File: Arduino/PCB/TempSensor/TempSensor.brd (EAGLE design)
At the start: 40.3 x 30.5 mm, 13 parts, among them IC1 DS18B20, U1 ATMEGA328-AU, X1 16Mhz

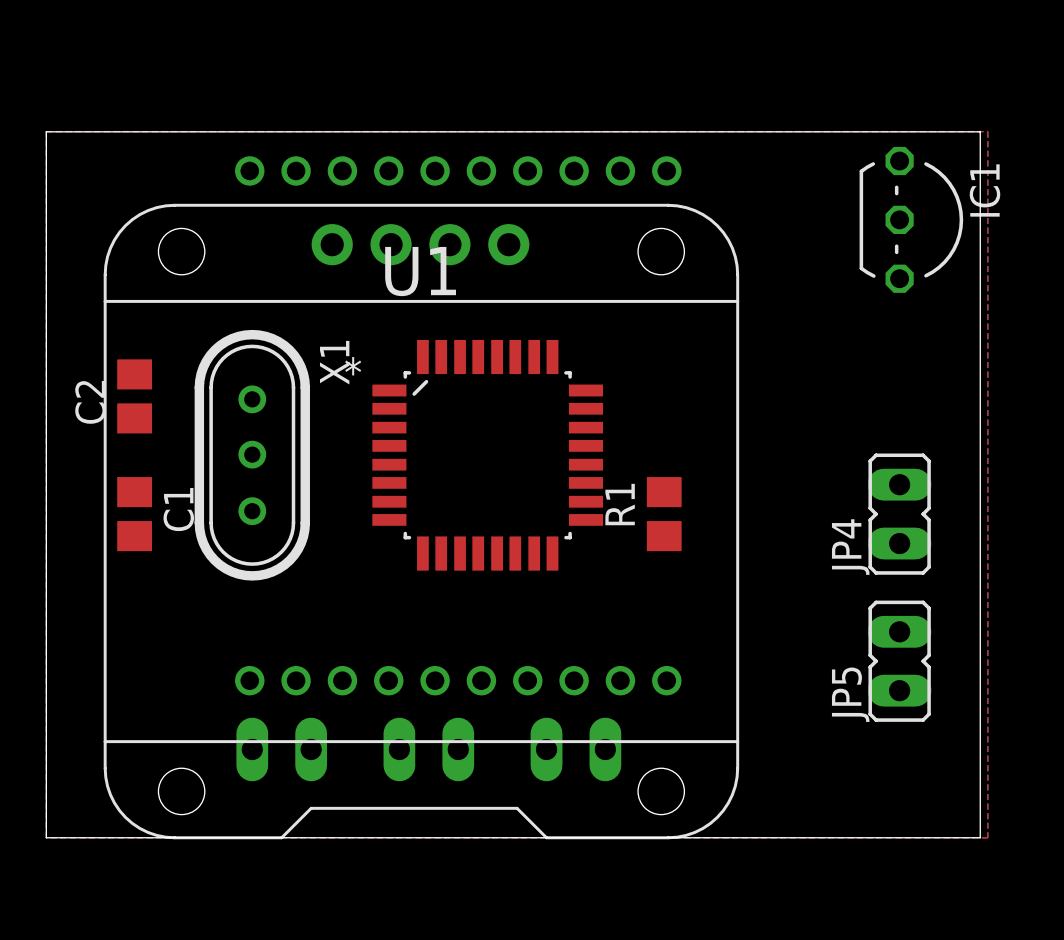
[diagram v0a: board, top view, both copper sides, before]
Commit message: sensor pcb
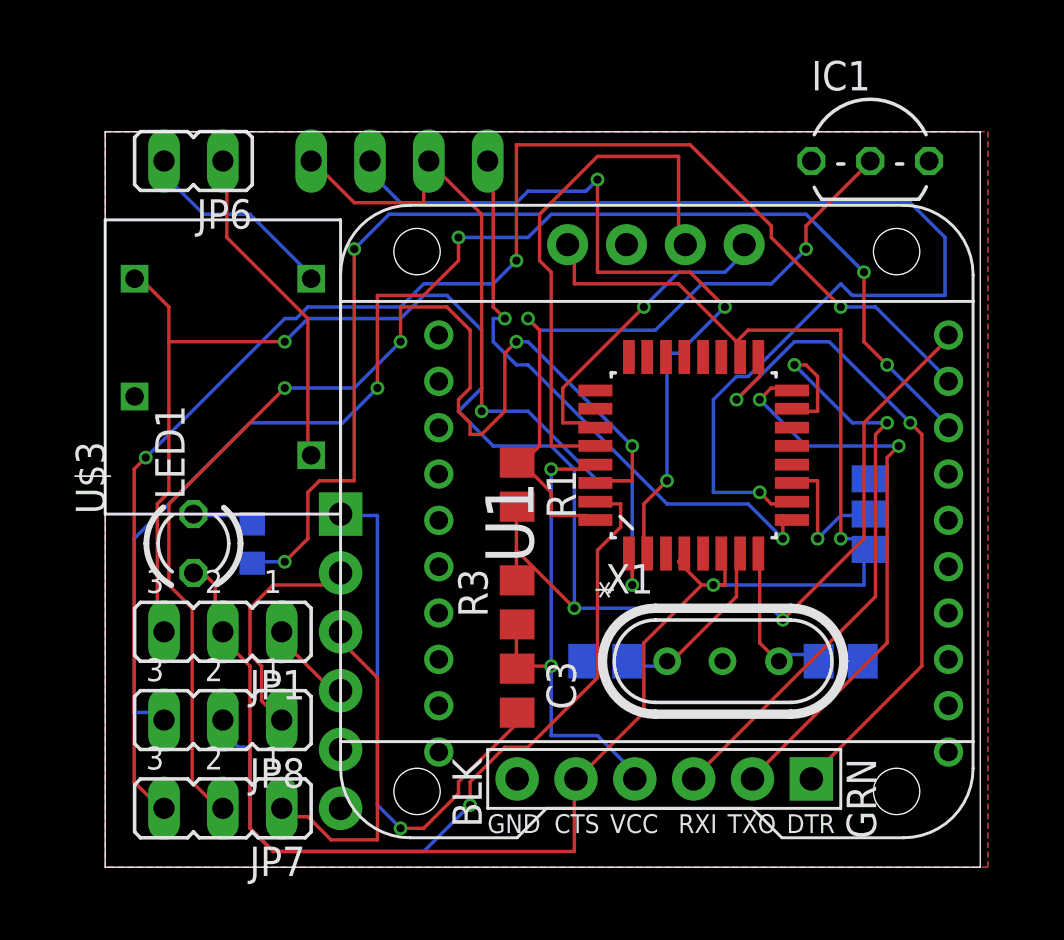
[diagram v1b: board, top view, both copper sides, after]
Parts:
- removed JP2, JP3: (no value), jumper:JP1
- added C3: 100n, rcl:C0805
- added J1, J2: FTDI_DEVICE, SparkFun-Connectors:FTDI_DEVICE_SIDE
- added JP6: (no value), jumper:JP1
- added JP7, JP8: (no value), jumper:JP2
- added LED1: 2mA, led:LED3MM
- added R2: 580, rcl:R0603
- added R3: 10k, rcl:R0805
- added SJ2: (no value), jumper:SJ_2
- added U$3: IE0503D, xp_power:XP_DIP
- JP1: device jumper:JP1 -> jumper:JP2
- R1: value (none) -> 4k7
- moved C1 31.1 mm to (63.5, 29.2), flipped to the bottom, turned to 180 degrees
- moved JP5 28.8 mm to (47.0, 50.8), flipped to the bottom, turned to 90 degrees
- moved JP4 28.5 mm to (41.9, 50.8), flipped to the bottom, turned to 90 degrees
- moved C2 23.3 mm to (53.3, 29.2), flipped to the bottom, turned to 180 degrees
- moved X1 22.2 mm to (58.4, 29.2), turned to 0 degrees
- moved XB1 11.4 mm to (57.1, 34.3), turned to 0 degrees
- moved U$2 10.2 mm to (55.9, 35.6)
- moved U1 8.89 mm to (57.1, 38.1), turned to 90 degrees
- moved R1 6.48 mm to (49.5, 36.8), turned to 270 degrees
- moved JP1 5.68 mm to (36.8, 30.5), flipped to the top, turned to 180 degrees
- moved IC1 2.84 mm to (64.8, 50.8), turned to 0 degrees
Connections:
- removed net N$3: JP3.2, XB1.1
- new net +5V: J1.P$4, JP1.1
- new net N$11: JP6.2, U$3.+VIN
- new net N$14: JP6.1, U$3.-VIN
- new net N$15: LED1.K, R2.2
- new net N$16: R2.1, U1.10
- new net N$17: SJ2.2, U1.11
- new net N$18: JP7.3, XB1.2
- new net N$19: JP8.3, XB1.3
- new net N$20: C3.1, J2.P$4, R3.1, U1.29
- new net N$21: C3.2, J1.P$1
- new net N$22: J2.P$3, U1.15
- new net N$23: J2.P$1, U1.17
- new net N$24: J2.P$2, U1.16
- new net VCC: J2.P$5, JP1.2, LED1.A, SJ2.1, U$2.VCC, U1.18, U1.4, U1.6
- net +3V3: now also JP1.3, R3.2, U$3.+VOUT, XB1.1; no longer JP3.1, U$2.VCC, U1.18, U1.4, U1.6
- net GND: now also J1.P$6, J2.P$6, SJ2.3, U$3.-VOUT
- net N$4: now also JP7.2; no longer JP1.1
- net N$5: now also JP8.2, U1.31; no longer JP1.2, XB1.2
- net N$6: now also J1.P$3, JP7.1; no longer JP2.1, XB1.3
- net N$7: now also J1.P$2, JP8.1; no longer JP2.2, U1.31
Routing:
- net VCC: track 0.00 -> 79.6 mm, vias 0 -> 2
- net +3V3: track 0.00 -> 78.5 mm, vias 0 -> 3
- net N$16: track 0.00 -> 66.4 mm, vias 0 -> 3
- net N$18: track 0.00 -> 63.7 mm, vias 0 -> 3
- net N$19: track 0.00 -> 58.4 mm, vias 0 -> 4
- net N$4: track 0.00 -> 52.0 mm, vias 0 -> 4
- net N$12: track 0.00 -> 34.0 mm, vias 0 -> 3
- net N$5: track 0.00 -> 33.9 mm, vias 0 -> 1
- net N$10: track 0.00 -> 32.8 mm, vias 0 -> 2
- net 1W: track 0.00 -> 30.4 mm, vias 0 -> 2
- net N$23: track 0.00 -> 29.8 mm, vias 0 -> 2
- net N$22: track 0.00 -> 27.7 mm, vias 0 -> 2
- net N$13: track 0.00 -> 26.0 mm, vias 0 -> 2
- net N$24: track 0.00 -> 25.4 mm, vias 0 -> 2
- net N$21: track 0.00 -> 23.2 mm, vias 0 -> 1
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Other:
- board size 40.3 x 30.5 mm -> 37.8 x 31.7 mm
